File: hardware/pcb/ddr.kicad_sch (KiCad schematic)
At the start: 1 part, among them U3 K4E6E304EC-EGCG

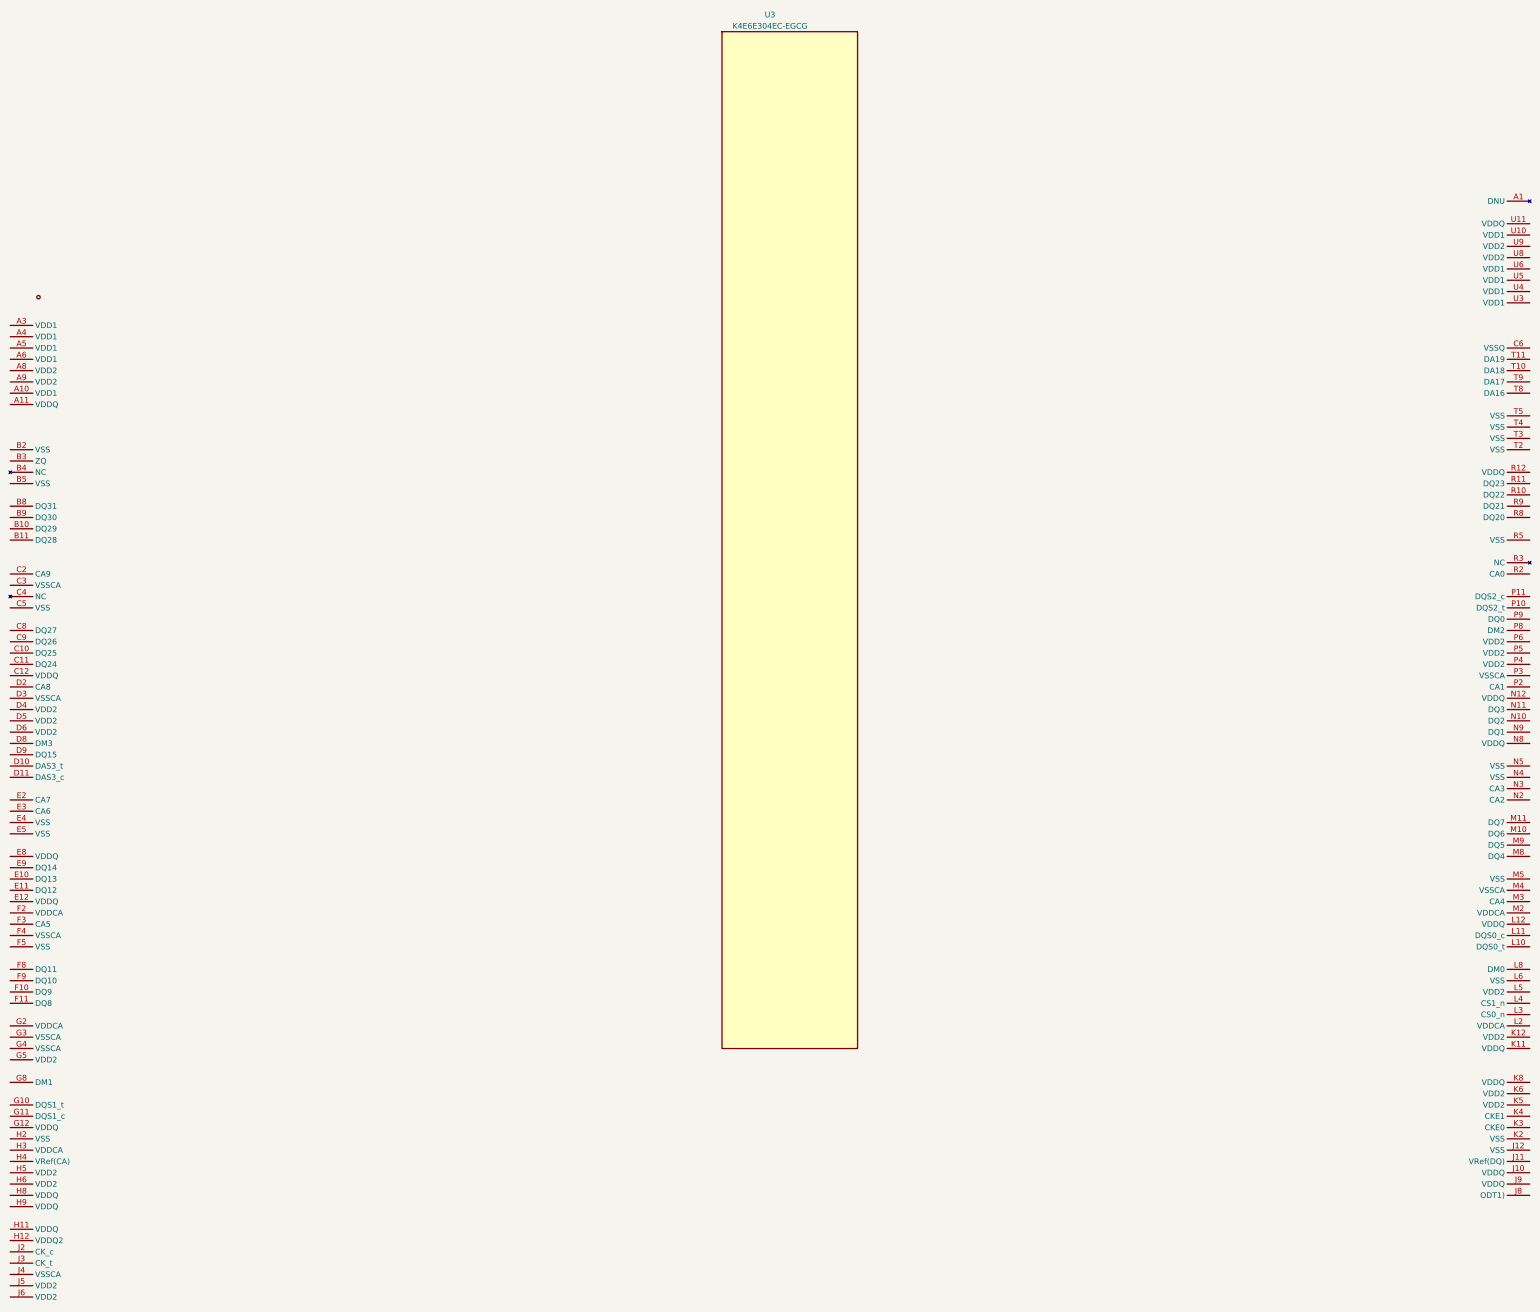
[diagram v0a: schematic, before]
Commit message: finished ddr symbol
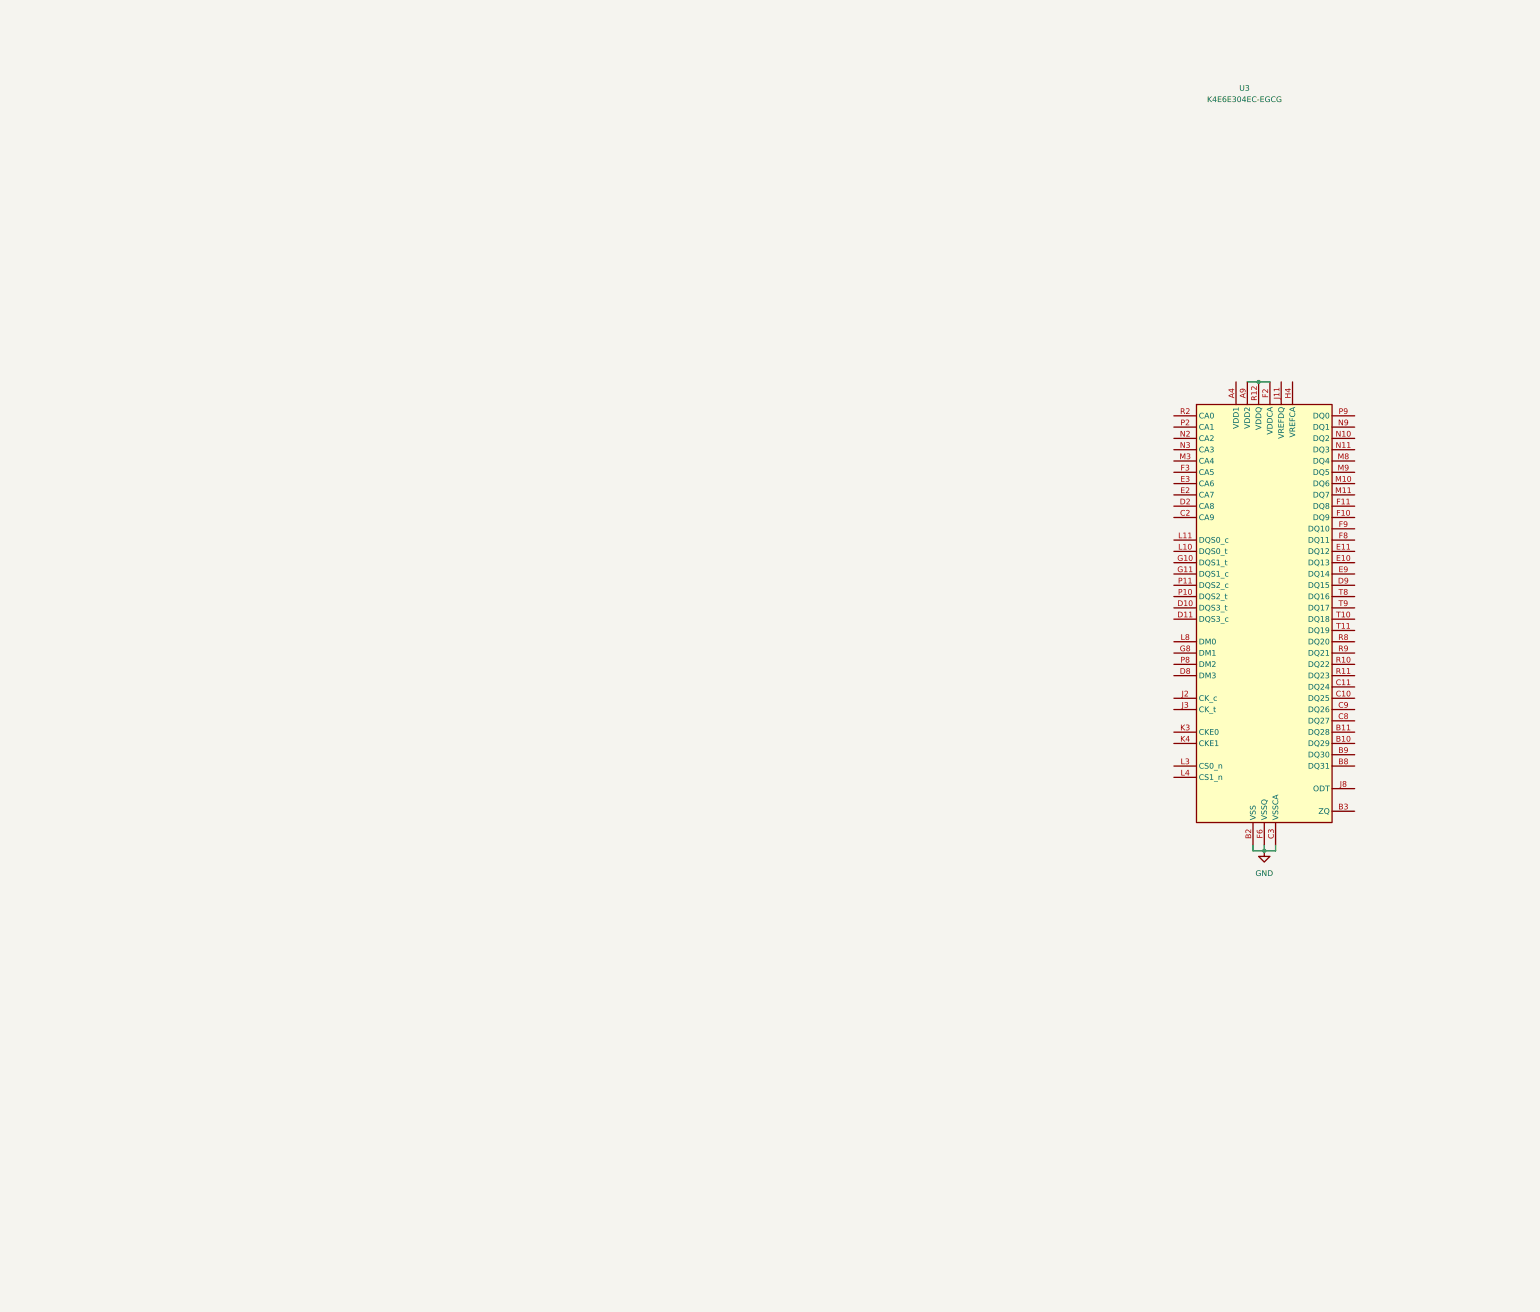
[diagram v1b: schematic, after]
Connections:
- net VSS is gone; now on net GND: U3.R4 (VSS), U3.R5 (VSS)
- net VSSQ is gone; now on net GND: U3.B12 (VSSQ), U3.B6 (VSSQ), U3.C6 (VSSQ), U3.D12 (VSSQ), U3.E6 (VSSQ), U3.F12 (VSSQ), U3.F6 (VSSQ), U3.G6 (VSSQ), U3.G9 (VSSQ), U3.H10 (VSSQ), U3.K10 (VSSQ), U3.L9 (VSSQ), U3.M12 (VSSQ), U3.M6 (VSSQ), U3.N6 (VSSQ), U3.P12 (VSSQ), U3.R6 (VSSQ), U3.T12 (VSSQ), U3.T6 (VSSQ)
- net VDD1: now reaches U3.A10 (VDD1)
- net VDD1: now also U3.A3 (VDD1), U3.A4 (VDD1), U3.A5 (VDD1), U3.A6 (VDD1), U3.U10 (VDD1), U3.U3 (VDD1), U3.U4 (VDD1), U3.U5 (VDD1), U3.U6 (VDD1)
- net VDD2: now reaches U3.A11 (VDDQ)
- net VDD2: now also U3.A8 (VDD2), U3.A9 (VDD2), U3.C12 (VDDQ), U3.D4 (VDD2), U3.D5 (VDD2), U3.D6 (VDD2), U3.E12 (VDDQ), U3.E8 (VDDQ), U3.F2 (VDDCA), U3.G12 (VDDQ), U3.G2 (VDDCA), U3.G5 (VDD2), U3.H11 (VDDQ), U3.H12 (VDDQ), U3.H3 (VDDCA), U3.H5 (VDD2), U3.H6 (VDD2), U3.H8 (VDDQ), U3.H9 (VDDQ), U3.J10 (VDDQ), U3.J5 (VDD2), U3.J6 (VDD2), U3.J9 (VDDQ), U3.K11 (VDDQ), U3.K12 (VDD2), U3.K5 (VDD2), U3.K6 (VDD2), U3.K8 (VDDQ), U3.L12 (VDDQ), U3.L2 (VDDCA), U3.L5 (VDD2), U3.M2 (VDDCA), U3.N12 (VDDQ), U3.N8 (VDDQ), U3.P4 (VDD2), U3.P5 (VDD2), U3.P6 (VDD2), U3.R12 (VDDQ), U3.U11 (VDDQ), U3.U8 (VDD2), U3.U9 (VDD2)
- net GND: now reaches U3.B2 (VSS)
- net GND: now also U3.B5 (VSS), U3.C3 (VSSCA), U3.C5 (VSS), U3.D3 (VSSCA), U3.E4 (VSS), U3.E5 (VSS), U3.F4 (VSSCA), U3.F5 (VSS), U3.G3 (VSSCA), U3.G4 (VSSCA), U3.H2 (VSS), U3.J12 (VSS), U3.J4 (VSSCA), U3.K2 (VSS), U3.L6 (VSS), U3.M4 (VSSCA), U3.M5 (VSS), U3.N4 (VSS), U3.N5 (VSS), U3.P3 (VSSCA), U3.T2 (VSS), U3.T3 (VSS), U3.T4 (VSS), U3.T5 (VSS)
- net at U3.B4 (NC): now also U3.C4 (NC), U3.K9 (NC), U3.R3 (NC)
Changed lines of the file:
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@@
 	(generator_version "10.0")
 	(paper "A4")
+	(junction
+		(at 135.89 33.02)
+		(diameter 0)
+		(color 0 0 0 0)
+	)
+	(junction
+		(at 137.16 138.43)
+		(diameter 0)
+		(color 0 0 0 0)
+	)
+	(wire
+		(pts
+			(xy 134.62 137.16) (xy 134.62 138.43)
+		)
+		(stroke
+			(width 0)
+			(type default)
+		)
+	)
+	(wire
+		(pts
+			(xy 139.7 138.43) (xy 137.16 138.43)
+		)
+		(stroke
+			(width 0)
+			(type default)
+		)
+	)
+	(wire
+		(pts
+			(xy 134.62 138.43) (xy 137.16 138.43)
+		)
+		(stroke
+			(width 0)
+			(type default)
+		)
+	)
+	(wire
+		(pts
+			(xy 135.89 33.02) (xy 138.43 33.02)
+		)
+		(stroke
+			(width 0)
+			(type default)
+		)
+	)
+	(wire
+		(pts
+			(xy 133.35 33.02) (xy 135.89 33.02)
+		)
+		(stroke
+			(width 0)
+			(type default)
+		)
+	)
+	(wire
+		(pts
+			(xy 139.7 137.16) (xy 139.7 138.43)
+		)
+		(stroke
+			(width 0)
+			(type default)
+		)
+	)
+	(wire
+		(pts
+			(xy 137.16 137.16) (xy 137.16 138.43)
+		)
+		(stroke
+			(width 0)
+			(type default)
+		)
 	)
 	(symbol
 		(lib_id "K4E6E304EC-EGCG:K4E6E304EC-EGCG")
-		(at 30.48 68.58 0)
+		(at 137.16 85.09 0)
 		(unit 1)
 		(body_style 1)
@@
 		(fields_autoplaced yes)
 		(property "Reference" "U3"
-			(at 26.035 -49.53 0)
+			(at 132.715 -33.02 0)
 			(show_name no)
 			(do_not_autoplace no)
@@
 		)
 		(property "Value" "K4E6E304EC-EGCG"
-			(at 26.035 -46.99 0)
+			(at 132.715 -30.48 0)
 			(show_name no)
 			(do_not_autoplace no)
@@
 		)
 		(property "Footprint" "K4E6E304EC-EGCG:FBGA-178_L11.5-W11.0_K4E6E304EC-TL"
-			(at 30.48 187.96 0)
+			(at 137.16 204.47 0)
 			(hide yes)
 			(show_name no)
@@
 		)
 		(property "Datasheet" "https://www.lcsc.com/datasheet/C2803256.pdf"
-			(at 30.48 190.5 0)
+			(at 137.16 207.01 0)
 			(hide yes)
 			(show_name no)
@@
 		)
 		(property "Description" ""
-			(at 30.48 68.58 0)
+			(at 137.16 85.09 0)
 			(hide yes)
 			(show_name no)
@@
 		)
 		(property "Manufacturer" "SAMSUNG(三星半导体)"
-			(at 30.48 193.04 0)
+			(at 137.16 209.55 0)
 			(hide yes)
 			(show_name no)
@@
 		)
 		(property "MPN" "K4E6E304EC-EGCG"
-			(at 30.48 195.58 0)
+			(at 137.16 212.09 0)
 			(hide yes)
 			(show_name no)
@@
 		)
 		(property "LCSC Part" "C2803256"
-			(at 30.48 198.12 0)
+			(at 137.16 214.63 0)
 			(hide yes)
 			(show_name no)
@@
 					(unit 1)
 				)
+			)
+		)
+	)
+	(symbol
+		(lib_id "power:GND")
+		(at 137.16 138.43 0)
+		(unit 1)
+		(body_style 1)
+		(exclude_from_sim no)
+		(in_bom yes)
+		(on_board yes)
+		(in_pos_files yes)
+		(dnp no)
+		(fields_autoplaced yes)
+		(property "Reference" "#PWR01"
+			(at 137.16 144.78 0)
+			(hide yes)
+			(show_name no)
+			(do_not_autoplace no)
+			(effects
+				(font
+					(size 1.27 1.27)
+				)
+			)
+		)
+		(property "Value" "GND"
+			(at 137.16 143.51 0)
+			(show_name no)
+			(do_not_autoplace no)
+			(effects
+				(font
+					(size 1.27 1.27)
+				)
+			)
+		)
+		(property "Footprint" ""
+			(at 137.16 138.43 0)
+			(hide yes)
+			(show_name no)
+			(do_not_autoplace no)
+			(effects
+				(font
+					(size 1.27 1.27)
+				)
+			)
+		)
+		(property "Datasheet" ""
+			(at 137.16 138.43 0)
+			(hide yes)
+			(show_name no)
+			(do_not_autoplace no)
+			(effects
+				(font
+					(size 1.27 1.27)
+				)
+			)
+		)
+		(property "Description" "Power symbol creates a global label with name \"GND\" , ground"
+			(at 137.16 138.43 0)
+			(hide yes)
+			(show_name no)
+			(do_not_autoplace no)
+			(effects
+				(font
+					(size 1.27 1.27)
+				)
+			)
+		)
+		(pin "1"
+		)
+		(instances
+			(project "meko"
+				(path "/da54f10a-146b-4941-a9c7-55c7173bb101/6a1996a1-d776-4235-b4ef-703258aa0c56"
+					(reference "#PWR01")
+					(unit 1)
+				)
